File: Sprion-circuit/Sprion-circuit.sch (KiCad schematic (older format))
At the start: 0 parts

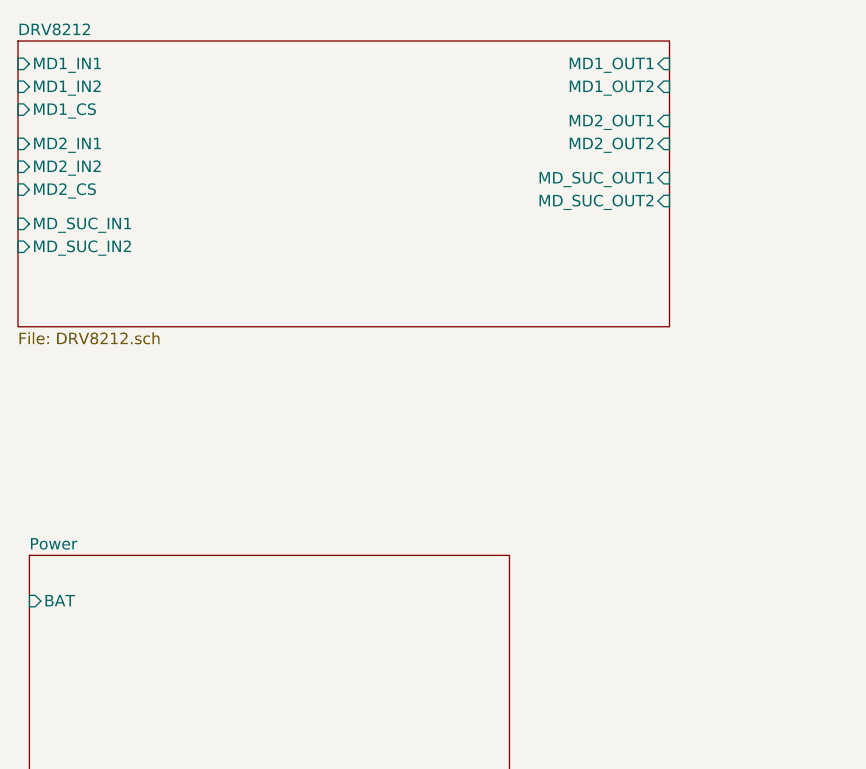
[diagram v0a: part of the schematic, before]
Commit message: Push, Push, Push
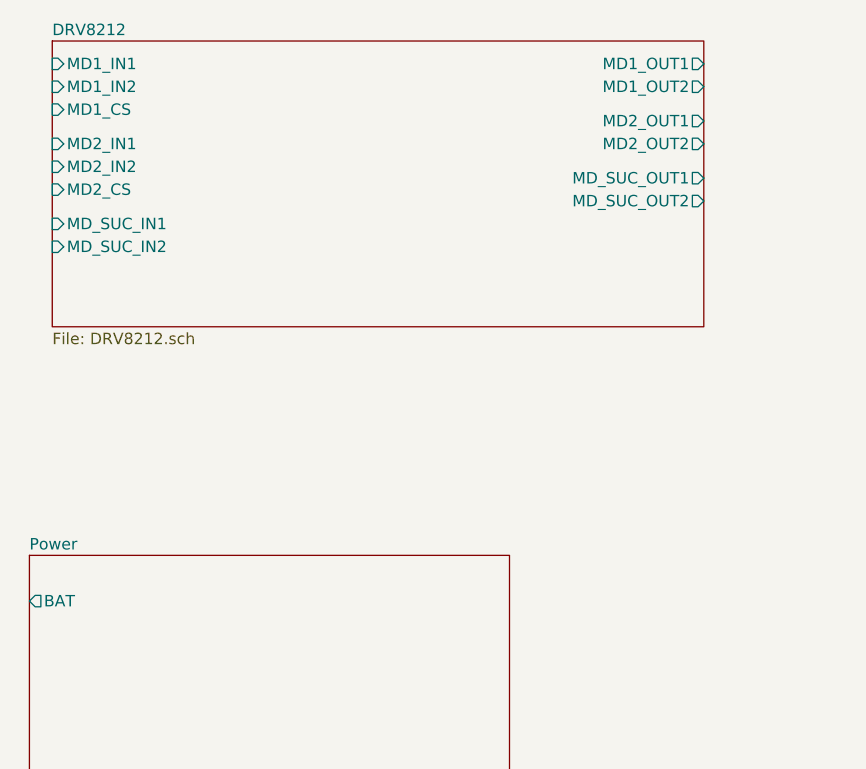
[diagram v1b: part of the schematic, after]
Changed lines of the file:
@@
 $EndDescr
 $Sheet
-S 1250 1500 2850 1250
+S 1400 1500 2850 1250
 U 60E26C28
 F0 "DRV8212" 50
 F1 "DRV8212.sch" 50
-F2 "MD1_IN1" I L 1250 1600 50
-F3 "MD1_IN2" I L 1250 1700 50
-F4 "MD1_OUT1" I R 4100 1600 50
-F5 "MD1_OUT2" I R 4100 1700 50
-F6 "MD1_CS" I L 1250 1800 50
-F7 "MD2_IN1" I L 1250 1950 50
-F8 "MD2_IN2" I L 1250 2050 50
-F9 "MD2_OUT1" I R 4100 1850 50
-F10 "MD2_OUT2" I R 4100 1950 50
-F11 "MD_SUC_IN1" I L 1250 2300 50
-F12 "MD_SUC_IN2" I L 1250 2400 50
-F13 "MD_SUC_OUT1" I R 4100 2100 50
-F14 "MD_SUC_OUT2" I R 4100 2200 50
-F15 "MD2_CS" I L 1250 2150 50
+F2 "MD1_IN1" I L 1400 1600 50
+F3 "MD1_IN2" I L 1400 1700 50
+F4 "MD1_OUT1" O R 4250 1600 50
+F5 "MD1_OUT2" O R 4250 1700 50
+F6 "MD1_CS" I L 1400 1800 50
+F7 "MD2_IN1" I L 1400 1950 50
+F8 "MD2_IN2" I L 1400 2050 50
+F9 "MD2_OUT1" O R 4250 1850 50
+F10 "MD2_OUT2" O R 4250 1950 50
+F11 "MD_SUC_IN1" I L 1400 2300 50
+F12 "MD_SUC_IN2" I L 1400 2400 50
+F13 "MD_SUC_OUT1" O R 4250 2100 50
+F14 "MD_SUC_OUT2" O R 4250 2200 50
+F15 "MD2_CS" I L 1400 2150 50
 $EndSheet
 $Sheet
@@
 F0 "Power" 50
 F1 "Power.sch" 50
-F2 "BAT" I L 1300 3950 50
+F2 "BAT" O L 1300 3950 50
 $EndSheet
 $Sheet
